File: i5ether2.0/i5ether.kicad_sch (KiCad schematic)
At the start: 14 parts, among them J2 Conn_02x05_Odd_Even, J3 1-406541-1, T2 HX5008

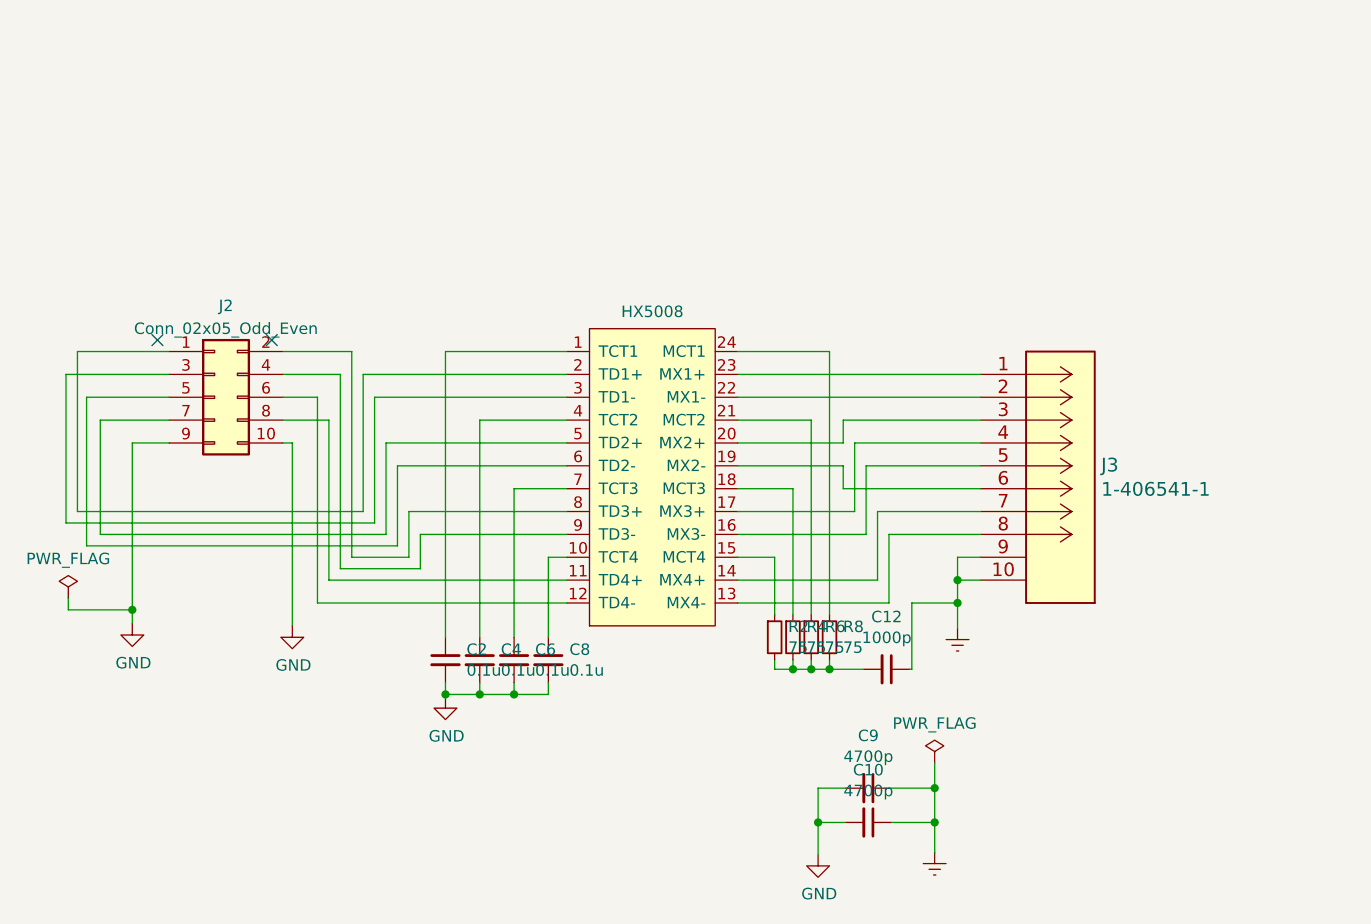
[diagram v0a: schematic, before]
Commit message: Modulos
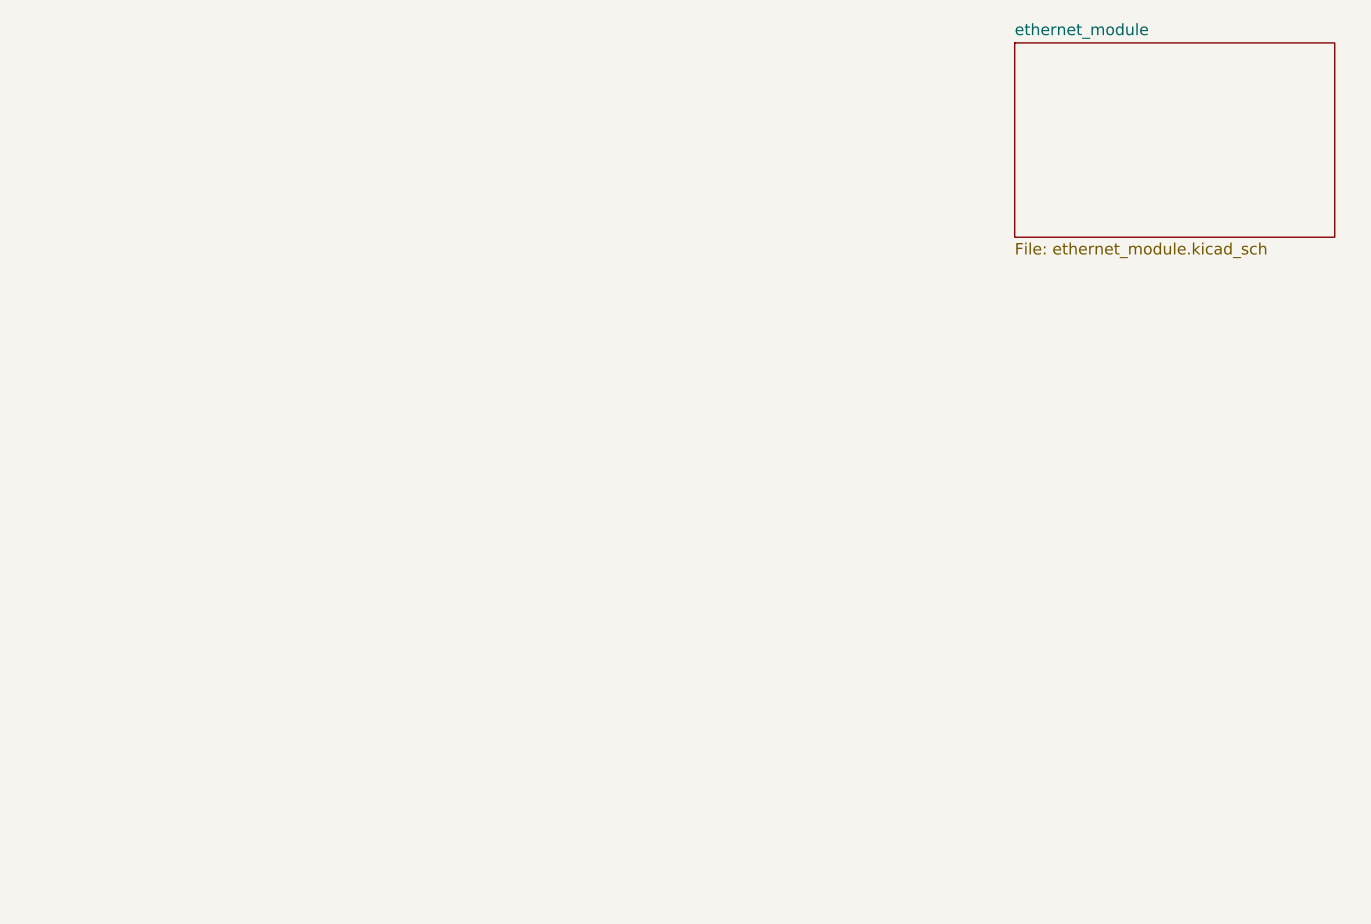
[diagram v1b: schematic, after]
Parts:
- removed C10, C9: 4700p, Resistor_SMD:R_1812_4532Metric, symbol Device:C_Small
- removed C12: 1000p, Capacitor_SMD:C_0402_1005Metric, symbol Device:C_Small
- removed C2, C4, C6, C8: 0.1u, Capacitor_SMD:C_0402_1005Metric, symbol Device:C_Small
- removed J2: Conn_02x05_Odd_Even, Connector_PinHeader_2.54mm:PinHeader_2x05_P2.54mm_Vertical, symbol Connector_Generic:Conn_02x05_Odd_Even
- removed J3: 1-406541-1, MJ406541:1-406541-1, symbol MJ406541:1-406541-1
- removed R2, R4, R6, R8: 75, Resistor_SMD:R_0402_1005Metric, symbol Device:R_Small
- removed T2: HX5008, HX5008:HX5008NL, symbol HX5008:HX5008
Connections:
- no-connect marks 2 -> 0
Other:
- added sheet ethernet_module (ethernet_module.kicad_sch)
